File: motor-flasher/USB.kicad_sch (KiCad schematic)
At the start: 16 parts, among them J1 USB4105-GF-A, J4 B2B-PH-K-S-GW, SW2 SS12D07VG4NSGAPA, U6 TPS61027DRCR

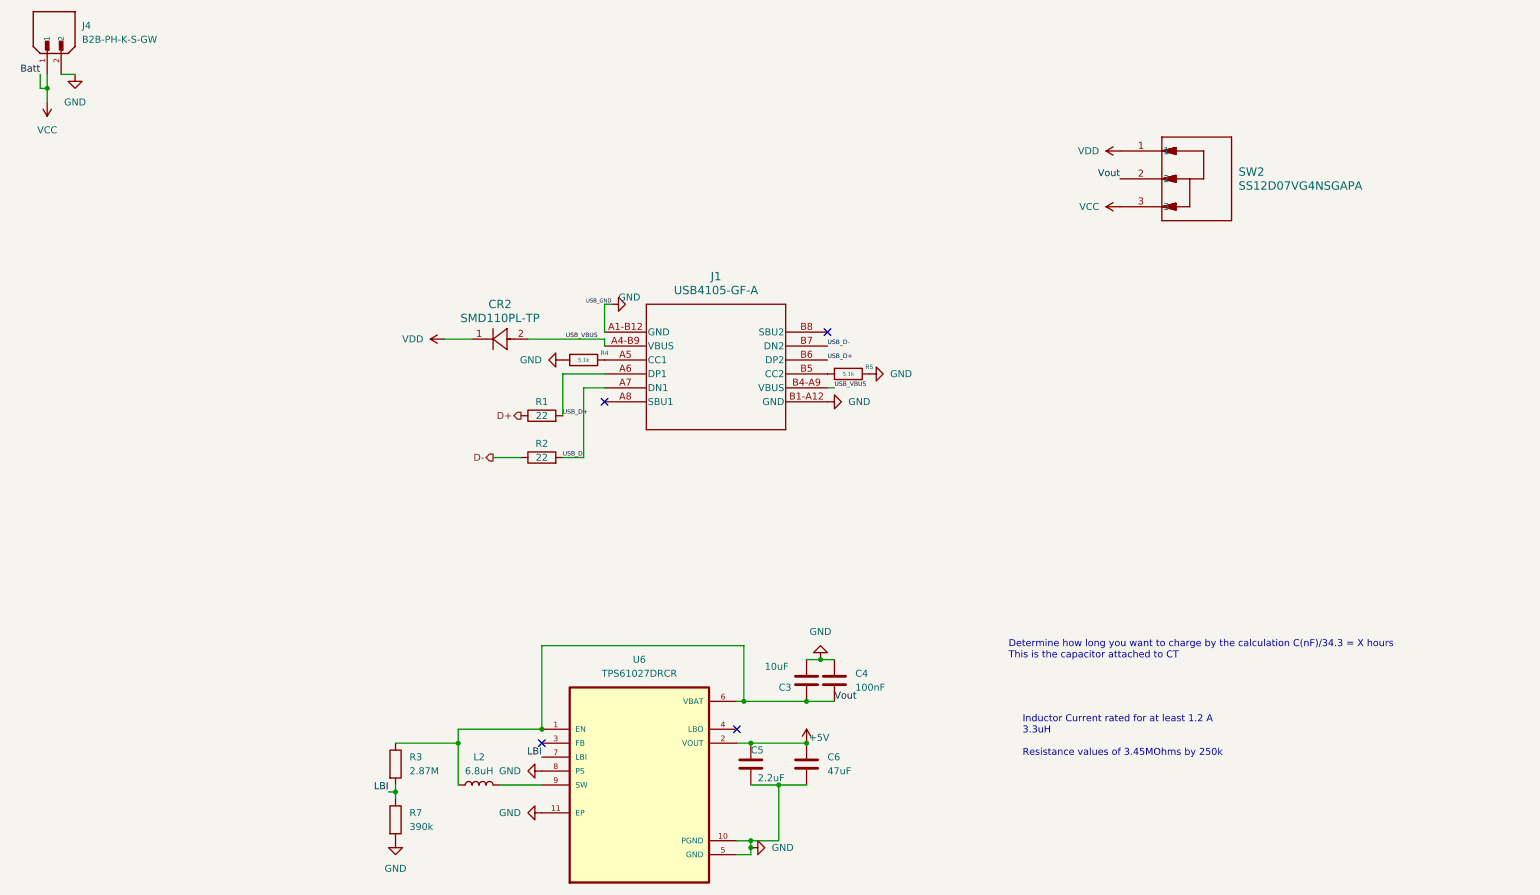
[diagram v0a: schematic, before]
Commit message: Beginning Layout Process
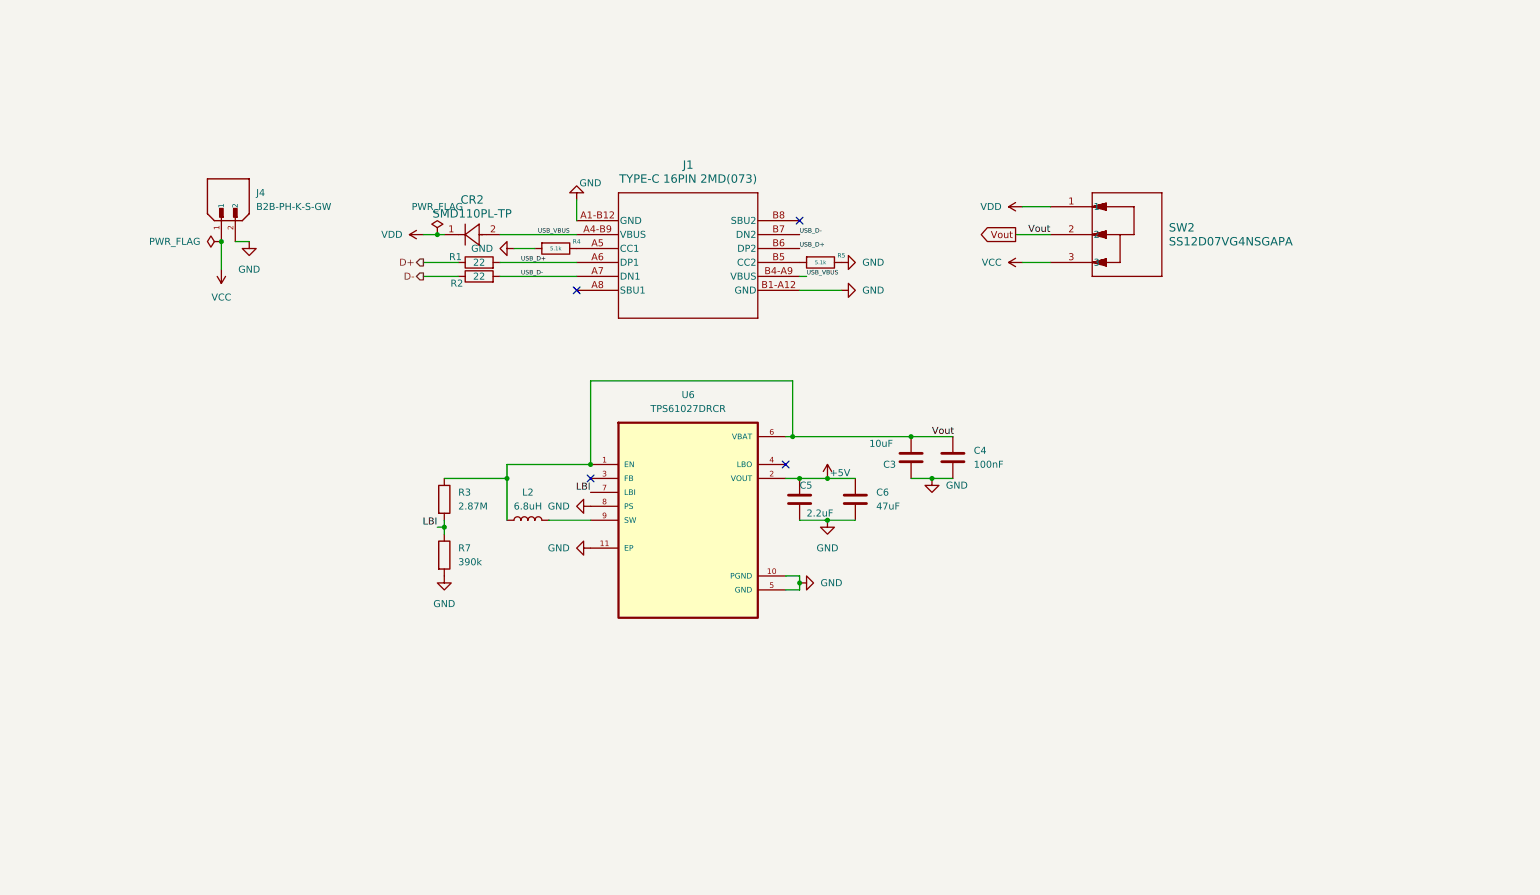
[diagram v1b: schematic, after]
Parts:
- CR2: footprint smd110:SOD-123FL_MCC -> Motor-Flasher:SOD-123FL_MCC
- J1: value USB4105-GF-A -> TYPE-C 16PIN 2MD(073); footprint revparts2:GCT_USB4105-GF-A -> Motor-Flasher:GCT_USB4105-GF-A
- J4: footprint revparts2:JST_B2B-XH-A -> Motor-Flasher:JST_B2B-XH-A
- L2: footprint revparts3:CDRH5D28RHP -> Motor-Flasher:CDRH5D28RHP
- SW2: footprint revparts2:SS12D07_CNK -> Motor-Flasher:SS12D07_CNK
- U6: footprint revparts2:VREG_V62_16624-01YE -> Motor-Flasher:VREG_V62_16624-01YE
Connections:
- net GND: now also C3.1, C4.1; no longer C3.2, C4.2
- net Vout: now also C3.2, C4.2; no longer C3.1, C4.1
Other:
- note removed: "Determine how long you want to charge by the calculation C(nF)/34.3 = X hours This is the capacitor attached to CT"
- note removed: "Inductor Current rated for at least 1.2 A 3.3uH Resistance values of 3.45MOhms by 250k"
- moved on the sheet: C3, C4, C5, C6, CR2, J1, J4, L2, R1, R2, R3, R4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
